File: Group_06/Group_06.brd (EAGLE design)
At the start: 97.8 x 83.8 mm, 29 parts, among them J1 POWER_JACKPTH_LOCK, U2 +12v

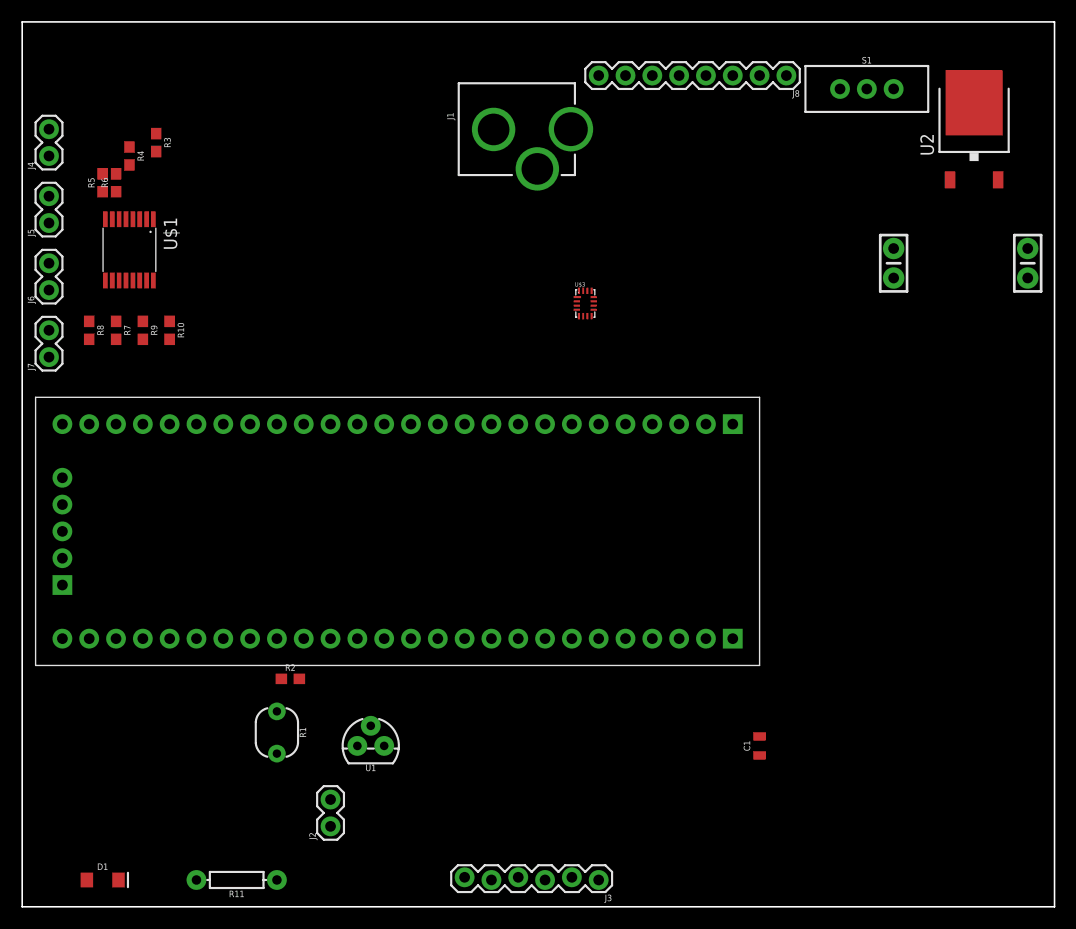
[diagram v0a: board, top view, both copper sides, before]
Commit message: Board Layout 1
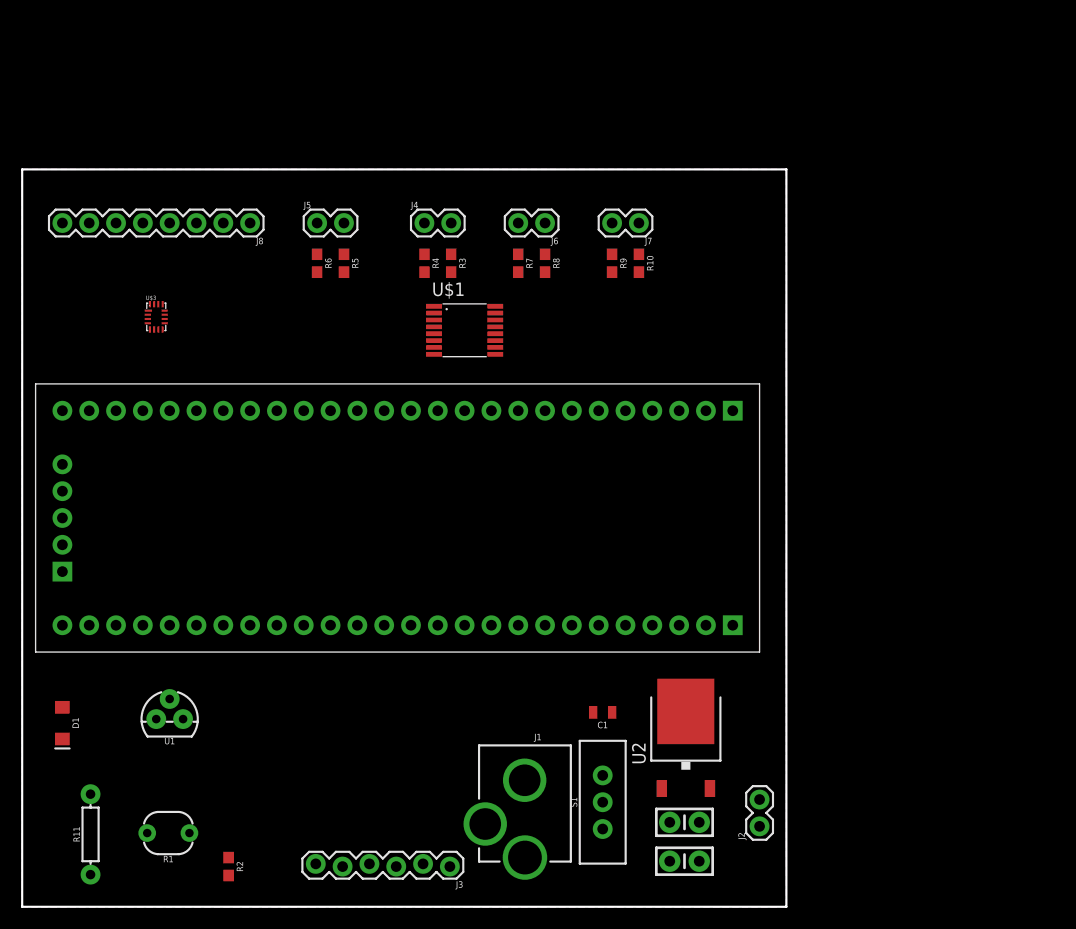
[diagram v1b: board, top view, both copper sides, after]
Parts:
- moved S1 72.0 mm to (55.0, 9.91), turned to 0 degrees
- moved U2 63.8 mm to (62.9, 16.0)
- moved C3 62.1 mm to (62.7, 8.00), turned to 180 degrees
- moved C2 60.0 mm to (62.7, 4.32), turned to 180 degrees
- moved J7 57.3 mm to (58.4, 64.8), turned to 180 degrees
- moved J1 55.9 mm to (47.6, 18.5), turned to 180 degrees
- moved J8 52.7 mm to (21.6, 64.8)
- moved J6 47.4 mm to (49.5, 64.8), turned to 180 degrees
- moved R10 44.9 mm to (58.4, 61.0)
- moved R9 44.9 mm to (55.9, 61.0)
- moved R8 43.6 mm to (49.5, 61.0)
- moved U$3 40.7 mm to (12.7, 55.9)
- moved J2 40.6 mm to (69.8, 7.62)
- moved R7 38.6 mm to (47.0, 61.0)
- moved J4 36.1 mm to (38.1, 64.8), turned to 0 degrees
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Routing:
- added copper zone on layer 16, net 5V
- added copper zone on layer 1, net GND
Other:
- board size 97.8 x 83.8 mm -> 72.4 x 69.8 mm
